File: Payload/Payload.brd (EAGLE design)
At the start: 40.6 x 63.2 mm, 22 parts, among them J1 XT60-M, U2 MIC29302WU-TRTO-263-5_MCH-M

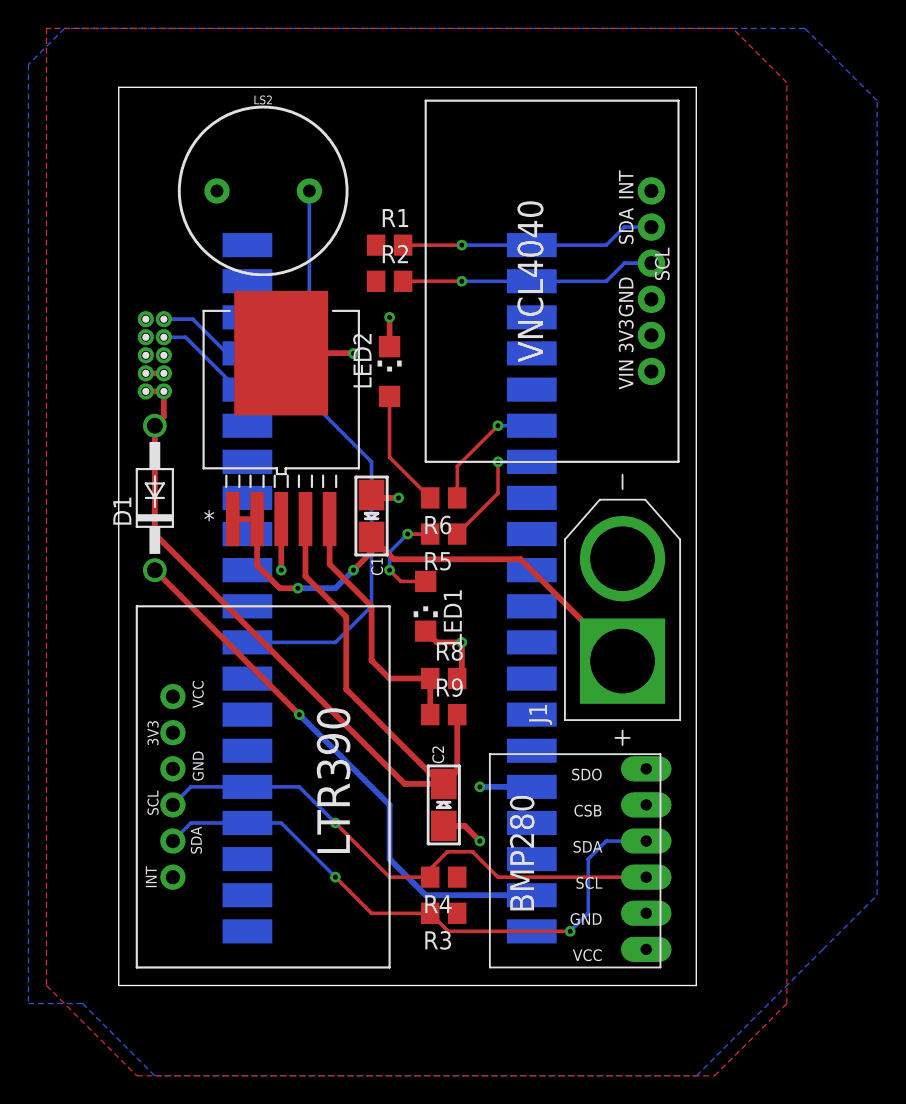
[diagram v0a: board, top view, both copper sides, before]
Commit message: payload pushed
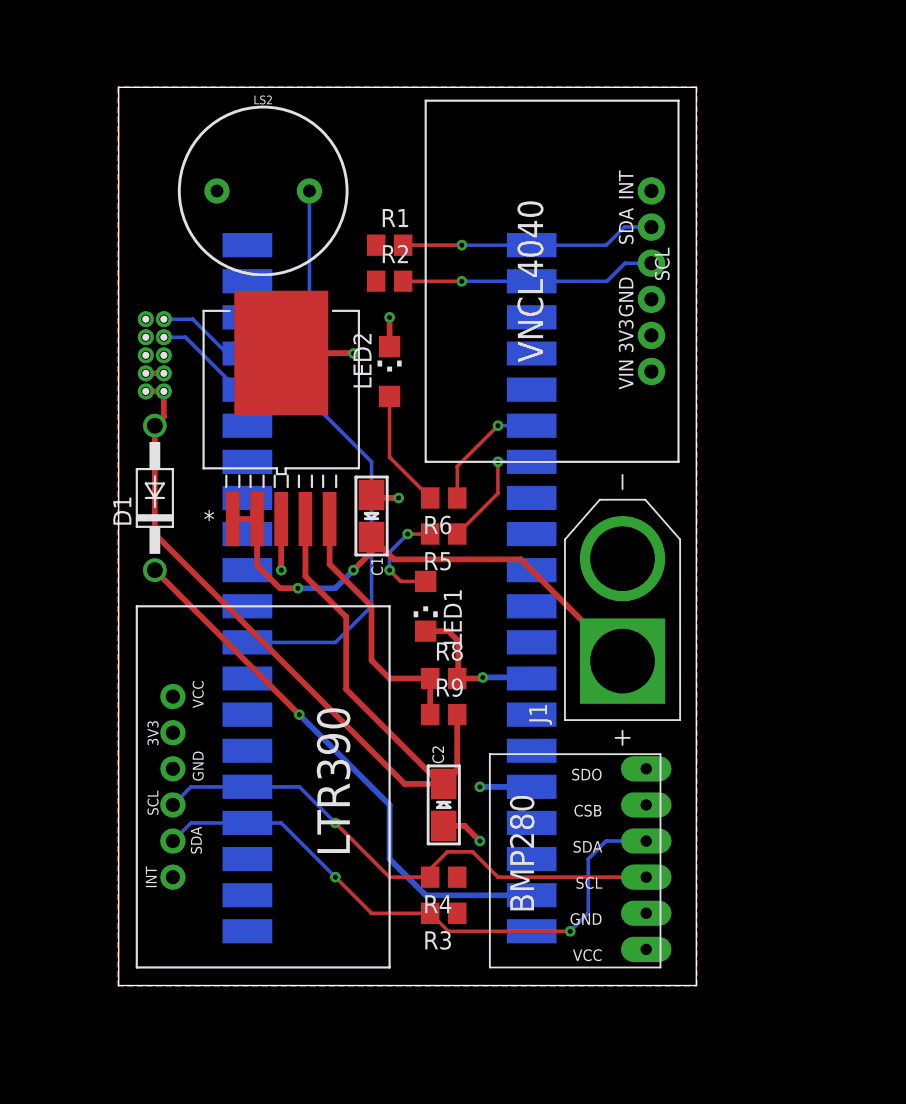
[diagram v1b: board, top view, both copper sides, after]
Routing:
- net GND: track 25.1 -> 30.1 mm
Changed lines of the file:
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@@
 <drawing>
 <settings>
-<setting alwaysvectorfont="yes"/>
+<setting alwaysvectorfont="no"/>
 <setting verticaltext="up"/>
 </settings>
-<grid distance="50" unitdist="mil" unit="mil" style="lines" multiple="1" display="yes" altdistance="5" altunitdist="mil" altunit="mil"/>
+<grid distance="1" unitdist="mil" unit="mil" style="lines" multiple="1" display="yes" altdistance="0.025" altunitdist="mil" altunit="mil"/>
 <layers>
 <layer number="1" name="Top" color="4" fill="1" visible="yes" active="yes"/>
@@
 <contactref element="U2" pad="6"/>
 <contactref element="LS2" pad="-"/>
-<polygon width="0.1524" layer="16">
-<vertex x="-6.35" y="64.77"/>
-<vertex x="-6.35" y="-1.27"/>
-<vertex x="-2.54" y="-1.27"/>
-<vertex x="2.54" y="-6.35"/>
-<vertex x="40.64" y="-6.35"/>
-<vertex x="49.53" y="2.54"/>
-<vertex x="53.34" y="6.35"/>
-<vertex x="53.34" y="62.23"/>
-<vertex x="48.26" y="67.31"/>
-<vertex x="3.81" y="67.31"/>
-<vertex x="-3.81" y="67.31"/>
-</polygon>
-<wire x1="23.81" y1="21.59" x2="24.13" y2="21.91" width="0.4064" layer="1"/>
-<wire x1="24.13" y1="21.91" x2="24.13" y2="24.13" width="0.4064" layer="1"/>
-<via x="24.13" y="24.13" extent="1-16" drill="0.35"/>
-<wire x1="21.59" y1="24.92" x2="22.38" y2="24.13" width="0.4064" layer="1"/>
-<wire x1="22.38" y1="24.13" x2="24.13" y2="24.13" width="0.4064" layer="1"/>
 <wire x1="11.43" y1="32.8041" x2="11.43" y2="29.21" width="0.4064" layer="1"/>
 <via x="11.43" y="29.21" extent="1-16" drill="0.35"/>
@@
 <wire x1="16.4846" y1="44.4754" x2="16.51" y2="44.45" width="0.4064" layer="1"/>
 <via x="16.51" y="44.45" extent="1-16" drill="0.35"/>
+<polygon width="0.1524" layer="16">
+<vertex x="-0.0762" y="-0.040640625"/>
+<vertex x="40.650159375" y="-0.040640625"/>
+<vertex x="40.6654" y="-0.0254"/>
+<vertex x="40.6654" y="63.1698"/>
+<vertex x="40.6146" y="63.2206"/>
+<vertex x="0" y="63.2206"/>
+<vertex x="-0.0762" y="63.1444"/>
+</polygon>
+<wire x1="21.59" y1="24.92" x2="23.1876" y2="24.92" width="0.4064" layer="1"/>
+<wire x1="23.1876" y1="24.92" x2="23.876" y2="24.2316" width="0.4064" layer="1"/>
+<wire x1="23.876" y1="24.2316" x2="23.876" y2="21.656" width="0.4064" layer="1"/>
+<wire x1="23.876" y1="21.656" x2="23.81" y2="21.59" width="0.4064" layer="1"/>
+<wire x1="23.81" y1="21.59" x2="25.527" y2="21.59" width="0.4064" layer="1"/>
+<wire x1="25.527" y1="21.59" x2="25.6032" y2="21.6662" width="0.4064" layer="1"/>
+<via x="25.6032" y="21.6662" extent="1-16" drill="0.35"/>
+<wire x1="25.6032" y1="21.6662" x2="28.9738" y2="21.6662" width="0.4064" layer="16"/>
+<wire x1="28.9738" y1="21.6662" x2="29.05" y2="21.59" width="0.4064" layer="16"/>
 </signal>
 <signal name="5V">
@@
 <contactref element="U1" pad="P$36"/>
 <contactref element="U$4" pad="VCC"/>
-<polygon width="0.1524" layer="1">
-<vertex x="-5.08" y="67.31"/>
-<vertex x="-5.08" y="0"/>
-<vertex x="1.27" y="-6.35"/>
-<vertex x="41.91" y="-6.35"/>
-<vertex x="46.99" y="-1.27"/>
-<vertex x="46.99" y="63.5"/>
-<vertex x="43.18" y="67.31"/>
-</polygon>
 <wire x1="29.05" y1="13.97" x2="25.4" y2="13.97" width="0.4064" layer="16"/>
 <via x="25.4" y="13.97" extent="1-16" drill="0.35"/>
+<polygon width="0.1524" layer="1">
+<vertex x="-0.0762" y="-0.0254"/>
+<vertex x="40.6146" y="-0.0254"/>
+<vertex x="40.6654" y="0.0254"/>
+<vertex x="40.6654" y="63.1698"/>
+<vertex x="40.64" y="63.1952"/>
+<vertex x="0" y="63.1952"/>
+<vertex x="-0.0762" y="63.119"/>
+</polygon>
 </signal>
 <signal name="SCL1">
@@
 <via x="24.13" y="49.53" extent="1-16" drill="0.35"/>
 <wire x1="24.13" y1="49.53" x2="29.05" y2="49.53" width="0.254" layer="16"/>
-<wire x1="37.465" y1="50.8" x2="35.56" y2="50.8" width="0.254" layer="16"/>
-<wire x1="35.56" y1="50.8" x2="34.29" y2="49.53" width="0.254" layer="16"/>
-<wire x1="34.29" y1="49.53" x2="29.05" y2="49.53" width="0.254" layer="16"/>
+<wire x1="37.465" y1="50.8" x2="35.6108" y2="50.8" width="0.254" layer="16"/>
+<wire x1="35.6108" y1="50.8" x2="34.3408" y2="49.53" width="0.254" layer="16"/>
+<wire x1="34.3408" y1="49.53" x2="29.05" y2="49.53" width="0.254" layer="16"/>
 </signal>
 <signal name="SDA1">
